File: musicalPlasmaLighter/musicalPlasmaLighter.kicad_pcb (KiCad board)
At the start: 2 copper layers, 50 x 9 mm, 19 parts, among them J1 USB_B_Micro, J2 Conn_01x01_Male, J3 Conn_01x01_Male, J4 Conn_01x01_Male, J5 Conn_01x01_Male, J6 Conn_01x01_Male, J7 Conn_01x01_Male, J8 Conn_01x01_Male, J9 Conn_01x01_Male, SW1 SW_Push, U1 ATtiny85-20SU, U2 LTC4054ES5-4.2, U3 74HCT00

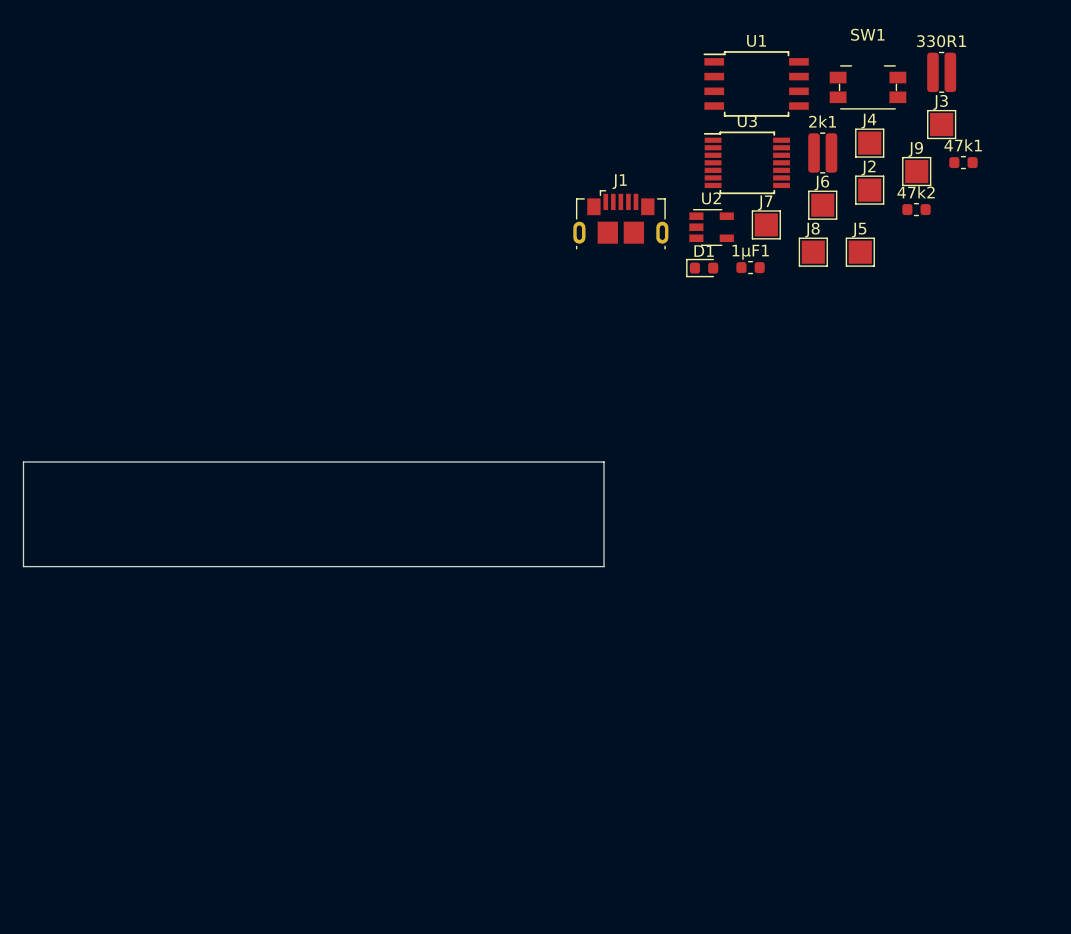
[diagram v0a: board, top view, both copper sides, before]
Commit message: updated pcb layout
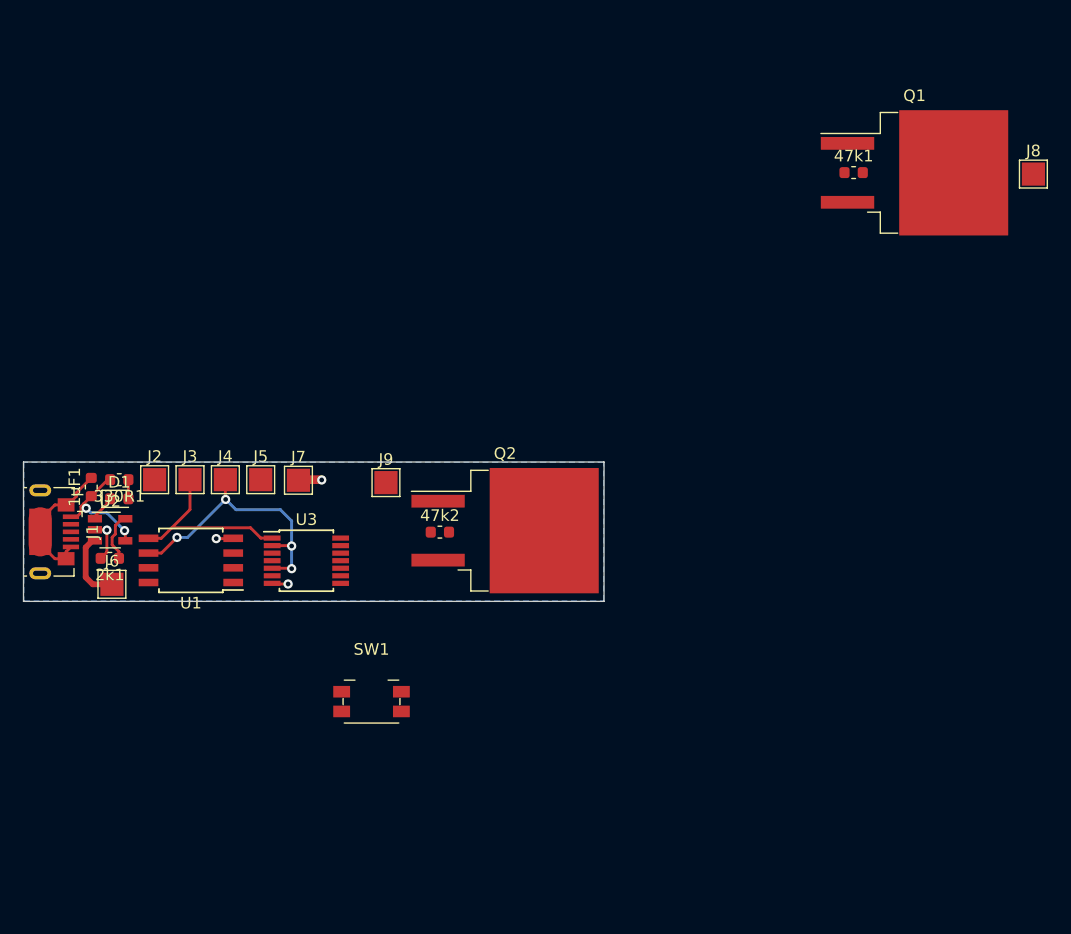
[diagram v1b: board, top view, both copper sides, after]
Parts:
- added Q1: 85N3LH5, Package_TO_SOT_SMD:TO-263-2, F.Cu at (160.2, 61.6)
- added Q2: 85N3LH5, Package_TO_SOT_SMD:TO-263-2, F.Cu at (124.9, 92.4)
- 2k1, 330R1: footprint Resistor_SMD:R_0612_1632Metric -> Resistor_SMD:R_0603_1608Metric
- moved 330R1 79.1 mm to (91.7, 88.0), turned to 180 degrees
- moved J3 71.7 mm to (97.8, 88.0)
- moved 2k1 70.7 mm to (90.9, 94.8), turned to 180 degrees
- moved J6 69.4 mm to (91.1, 97.0)
- moved SW1 68.1 mm to (113.4, 107.1)
- moved J2 66.5 mm to (94.7, 88.0)
- moved U1 63.8 mm to (97.9, 95.0), turned to 180 degrees
- moved J4 62.7 mm to (100.8, 88.0)
- moved 1µF1 59.9 mm to (89.3, 88.6), turned to 90 degrees
- moved U2 58.0 mm to (90.9, 92.3)
- moved J1 55.8 mm to (86.1, 92.5), turned to 270 degrees
- moved J5 55.3 mm to (103.9, 88.0)
- moved D1 54.2 mm to (91.7, 89.7)
- moved J9 53.0 mm to (114.7, 88.3)
- moved U3 51.2 mm to (107.8, 95.0)
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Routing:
- net Vmod: track 0.00 -> 24.2 mm, vias 0 -> 4
- net GND: track 0.00 -> 21.0 mm, vias 0 -> 4
- net Vcarrier: track 0.00 -> 16.2 mm
- net VCC: track 0.00 -> 10.5 mm, vias 0 -> 2
- net Net-(J6-Pad1): track 0.00 -> 6.11 mm
- net Net-(2k1-Pad1): track 0.00 -> 4.30 mm
- net Net-(D1-Pad1): track 0.00 -> 2.35 mm
- net Net-(330R1-Pad1): track 0.00 -> 1.65 mm
- added copper zone on B.Cu, net GND
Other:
- board size 50 x 9 mm -> 50 x 12 mm

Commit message: edited pcb
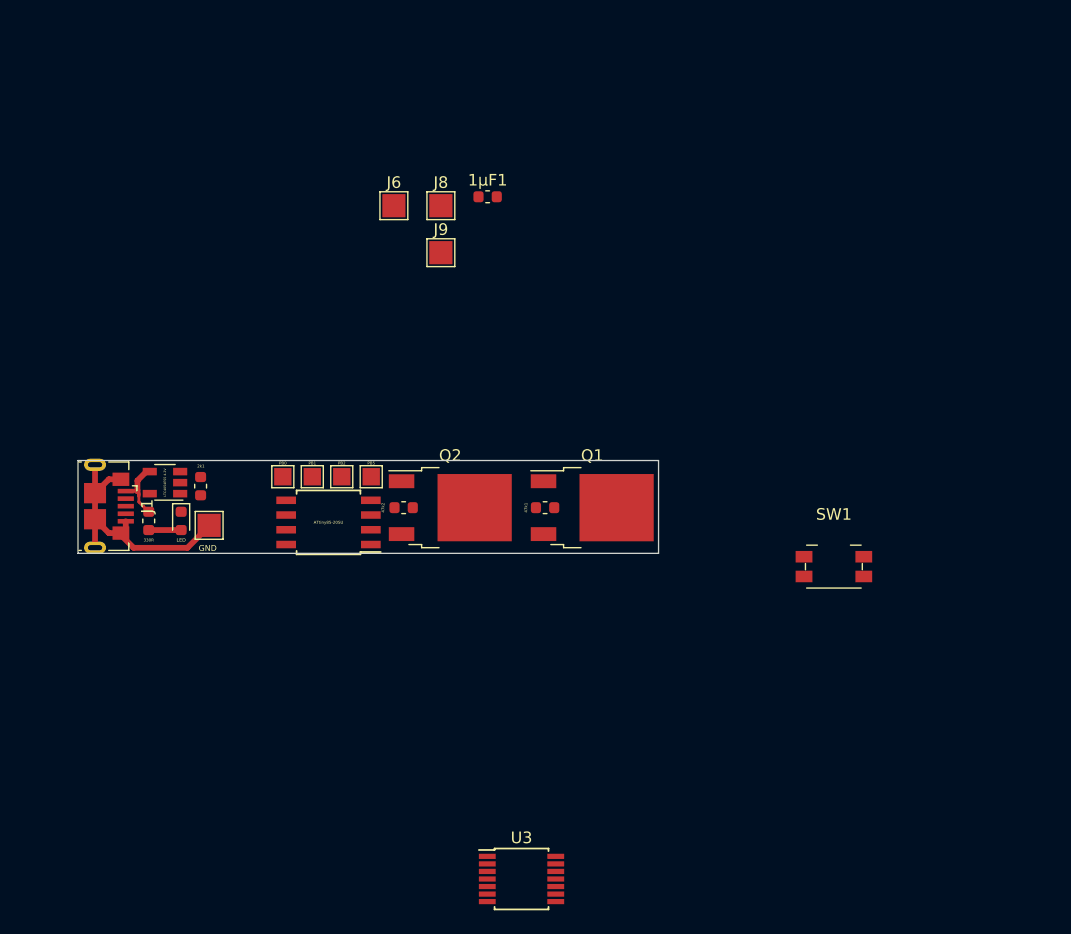
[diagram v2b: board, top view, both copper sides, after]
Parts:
- removed 330R1: R, Resistor_SMD:R_0603_1608Metric
- removed D1: LED, LED_SMD:LED_0603_1608Metric
- removed J2, J3, J4, J5, J7: Conn_01x01_Male, TestPoint:TestPoint_Pad_2.0x2.0mm
- removed U1: ATtiny85-20SU, Package_SO:SOIJ-8_5.3x5.3mm_P1.27mm
- removed U2: LTC4054ES5-4.2, Package_TO_SOT_SMD:TSOT-23-5
- added 330R: R, Resistor_SMD:R_0603_1608Metric, F.Cu at (94.2, 91.6)
- added ATtiny85-20SU: ATtiny85-20SU, Package_SO:SOIJ-8_5.3x5.3mm_P1.27mm, F.Cu at (109.7, 91.7)
- added GND: Conn_01x01_Male, TestPoint:TestPoint_Pad_2.0x2.0mm, F.Cu at (99.4, 91.9)
- added LED: LED, LED_SMD:LED_0603_1608Metric, F.Cu at (97.0, 91.6)
- added LTC4054ES5 4.2V: LTC4054ES5-4.2, Package_TO_SOT_SMD:TSOT-23-5, F.Cu at (95.6, 88.3)
- added PB0: Conn_01x01_Male, TestPoint:TestPoint_Pad_1.5x1.5mm, F.Cu at (105.8, 87.8)
- added PB1: Conn_01x01_Male, TestPoint:TestPoint_Pad_1.5x1.5mm, F.Cu at (108.3, 87.8)
- added PB2: Conn_01x01_Male, TestPoint:TestPoint_Pad_1.5x1.5mm, F.Cu at (110.9, 87.8)
- added PB5: Conn_01x01_Male, TestPoint:TestPoint_Pad_1.5x1.5mm, F.Cu at (113.4, 87.8)
- Q1, Q2: footprint Package_TO_SOT_SMD:TO-263-2 -> Package_TO_SOT_SMD:TO-252-2
- moved J8 51.1 mm to (119.4, 64.4)
- moved 1µF1 42.3 mm to (123.4, 63.6), turned to 0 degrees
- moved SW1 41.5 mm to (153.3, 95.5)
- moved J6 40.7 mm to (115.4, 64.4)
- moved Q1 40.1 mm to (132.5, 90.4)
- moved 47k1 39.3 mm to (128.4, 90.4)
- moved U3 33.1 mm to (126.4, 122.4)
- moved J9 20.4 mm to (119.4, 68.4)
- moved 2k1 10.00 mm to (98.7, 88.6), turned to 90 degrees
- moved J1 5.22 mm to (90.8, 90.3)
- moved Q2 5.12 mm to (120.2, 90.4)
- moved 47k2 3.77 mm to (116.2, 90.4)
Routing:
- net Vmod: track 24.2 -> 0.00 mm, vias 4 -> 0
- net Vcarrier: track 16.2 -> 0.00 mm
- net Net-(J6-Pad1): track 6.11 -> 0.00 mm
- net VCC: track 10.5 -> 5.89 mm, vias 2 -> 0
- net Net-(2k1-Pad1): track 4.30 -> 0.00 mm
- net Net-(D1-Pad1): track 2.35 -> 0.00 mm
- net GND: track 21.0 -> 22.8 mm, vias 4 -> 0
- net Net-(330R1-Pad1): track 1.65 -> 2.79 mm
- removed copper zone on B.Cu, net GND
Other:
- board size 50 x 12 mm -> 50 x 8 mm
- net class PWR added: clearance 0.2, trace_width 2, via_dia 1.5, via_drill 1
